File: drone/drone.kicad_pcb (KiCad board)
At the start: 2 copper layers, 50.8 x 50.8 mm, 28 parts, among them J1 Conn_01x03, J2 Conn_02x03_Top_Bottom, J3 Conn_01x02, J4 Conn_01x02, J5 Conn_01x02, J6 Conn_01x02, Q1 Si2319CDS, Q2 Si2319CDS, Q3 Si2319CDS, Q4 Si2319CDS, U1 ATmega328P-A, U2 MPU-6050, U3 DWM1000

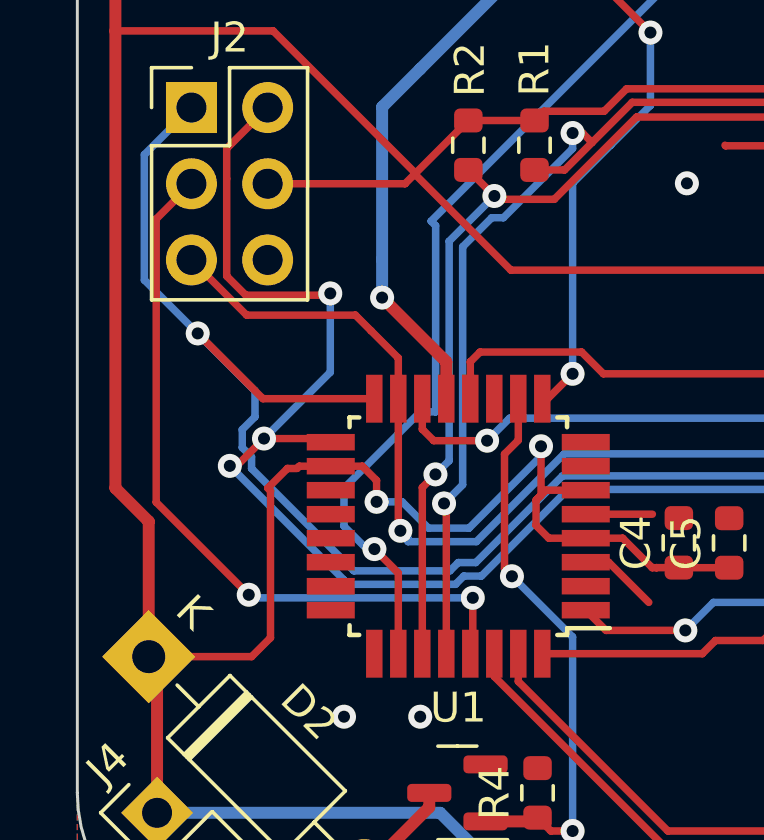
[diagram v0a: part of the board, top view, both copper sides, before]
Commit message: add reamde
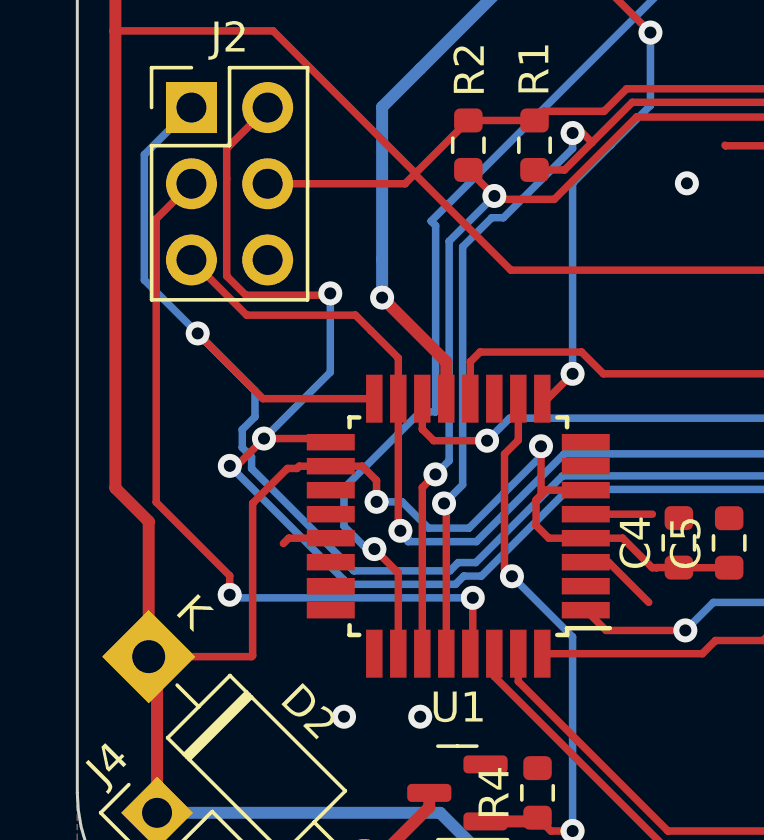
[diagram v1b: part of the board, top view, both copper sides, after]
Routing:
- net GND: track 14.3 -> 15.9 mm
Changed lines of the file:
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@@
   (segment (start 97.81 100.35) (end 97.79 100.33) (width 0.25) (layer "F.Cu") (net 36))
   (segment (start 93.15 112.63) (end 95.3702 112.63) (width 0.25) (layer "F.Cu") (net 36))
+  (segment (start 84.65 113.43) (end 83.246836 113.43) (width 0.25) (layer "F.Cu") (net 36))
   (segment (start 99.65 100.35) (end 97.81 100.35) (width 0.25) (layer "F.Cu") (net 36))
   (segment (start 100.825 105.41) (end 101.35 104.885) (width 0.25) (layer "F.Cu") (net 36))
   (segment (start 102.35 103.55) (end 102.35 104.040685) (width 0.25) (layer "F.Cu") (net 36))
+  (segment (start 83.246836 113.43) (end 83.068375 113.608461) (width 0.25) (layer "F.Cu") (net 36))
   (segment (start 103.15 106.4) (end 102.87 106.68) (width 0.25) (layer "F.Cu") (net 36))
   (segment (start 93.91 114.23) (end 95.25 115.57) (width 0.25) (layer "F.Cu") (net 36))
@@
   (segment (start 84.6328 107.8992) (end 82.423 110.109) (width 0.25) (layer "B.Cu") (net 38))
   (segment (start 89.3826 115.4176) (end 89.3826 117.1974) (width 0.25) (layer "F.Cu") (net 39))
-  (segment (start 78.83 102.79) (end 78.83 112.231) (width 0.25) (layer "F.Cu") (net 39))
-  (segment (start 78.83 112.231) (end 81.915 115.316) (width 0.25) (layer "F.Cu") (net 39))
   (segment (start 89.3826 117.1974) (end 89.3 117.28) (width 0.25) (layer "F.Cu") (net 39))
-  (segment (start 80.005 101.615) (end 78.83 102.79) (width 0.25) (layer "F.Cu") (net 39))
+  (segment (start 78.83 102.79) (end 80.005 101.615) (width 0.25) (layer "F.Cu") (net 39))
+  (segment (start 78.83 112.231) (end 78.83 102.79) (width 0.25) (layer "F.Cu") (net 39))
+  (segment (start 81.28 114.681) (end 78.83 112.231) (width 0.25) (layer "F.Cu") (net 39))
+  (segment (start 81.28 115.316) (end 81.28 114.681) (width 0.25) (layer "F.Cu") (net 39))
   (via (at 89.3826 115.4176) (size 0.8) (drill 0.4) (layers "F.Cu" "B.Cu") (net 39))
-  (via (at 81.915 115.316) (size 0.8) (drill 0.4) (layers "F.Cu" "B.Cu") (net 39))
-  (segment (start 82.0166 115.4176) (end 89.3826 115.4176) (width 0.25) (layer "B.Cu") (net 39))
-  (segment (start 81.915 115.316) (end 82.0166 115.4176) (width 0.25) (layer "B.Cu") (net 39))
+  (via (at 81.28 115.316) (size 0.8) (drill 0.4) (layers "F.Cu" "B.Cu") (net 39))
+  (segment (start 81.3816 115.4176) (end 89.3826 115.4176) (width 0.25) (layer "B.Cu") (net 39))
+  (segment (start 81.28 115.316) (end 81.3816 115.4176) (width 0.25) (layer "B.Cu") (net 39))
   (segment (start 117.390235 124.681275) (end 115.91896 123.21) (width 0.4) (layer "F.Cu") (net 40))
   (segment (start 103.55 102.85) (end 104.985 102.85) (width 0.25) (layer "F.Cu") (net 40))
@@
   (segment (start 90.6526 104.4956) (end 87.4739 101.3169) (width 0.25) (layer "F.Cu") (net 40))
   (segment (start 95.3638 114.4138) (end 94.38 113.43) (width 0.25) (layer "F.Cu") (net 40))
-  (segment (start 83.205 111.105) (end 82.55 111.76) (width 0.25) (layer "F.Cu") (net 40))
   (segment (start 91.656852 110.36615) (end 91.656852 112.000348) (width 0.25) (layer "F.Cu") (net 40))
+  (segment (start 82.044987 117.345013) (end 82.011634 117.378366) (width 0.25) (layer "F.Cu") (net 40))
   (segment (start 94.38 113.43) (end 93.15 113.43) (width 0.25) (layer "F.Cu") (net 40))
   (segment (start 117.057898 78.957898) (end 115.242492 77.142492) (width 0.4) (layer "F.Cu") (net 40))
   (segment (start 78.642492 80.760244) (end 78.837057 80.565679) (width 0.4) (layer "F.Cu") (net 40))
-  (segment (start 84.65 111.03) (end 83.6 111.03) (width 0.25) (layer "F.Cu") (net 40))
-  (segment (start 83.6 111.03) (end 83.525 111.105) (width 0.25) (layer "F.Cu") (net 40))
   (segment (start 91.8272 111.83) (end 91.4908 112.1664) (width 0.25) (layer "F.Cu") (net 40))
   (segment (start 106.167663 104.521) (end 105.8926 104.521) (width 0.25) (layer "F.Cu") (net 40))
@@
   (segment (start 119.6588 97.435) (end 119.6588 95.3) (width 0.25) (layer "F.Cu") (net 40))
   (segment (start 117.3557 79.2557) (end 117.057898 78.957898) (width 0.4) (layer "F.Cu") (net 40))
+  (segment (start 82.044987 112.265013) (end 82.044987 117.345013) (width 0.25) (layer "F.Cu") (net 40))
   (segment (start 78.580684 117.378366) (end 78.580684 112.870684) (width 0.4) (layer "F.Cu") (net 40))
   (segment (start 106.205996 97.975) (end 107.6706 99.439604) (width 0.25) (layer "F.Cu") (net 40))
+  (segment (start 83.205 111.105) (end 82.044987 112.265013) (width 0.25) (layer "F.Cu") (net 40))
   (segment (start 115.242492 77.142492) (end 80.337508 77.142492) (width 0.4) (layer "F.Cu") (net 40))
-  (segment (start 82.55 111.76) (end 82.64 111.85) (width 0.25) (layer "F.Cu") (net 40))
   (segment (start 77.47 96.52) (end 77.47 86.999189) (width 0.4) (layer "F.Cu") (net 40))
   (segment (start 100.85 104.3566) (end 100.711 104.4956) (width 0.25) (layer "F.Cu") (net 40))
-  (segment (start 82.64 111.85) (end 82.64 116.75) (width 0.25) (layer "F.Cu") (net 40))
-  (segment (start 82.011634 117.378366) (end 78.580684 117.378366) (width 0.25) (layer "F.Cu") (net 40))
   (segment (start 116.8588 95.3) (end 116.8588 97.6818) (width 0.25) (layer "F.Cu") (net 40))
   (segment (start 82.7278 96.52) (end 77.47 96.52) (width 0.25) (layer "F.Cu") (net 40))
   (segment (start 78.74 78.74) (end 78.837057 78.837057) (width 0.4) (layer "F.Cu") (net 40))
   (segment (start 122.644025 124.436286) (end 117.635224 124.436286) (width 0.4) (layer "F.Cu") (net 40))
-  (segment (start 83.525 111.105) (end 83.205 111.105) (width 0.25) (layer "F.Cu") (net 40))
   (segment (start 91.4908 113.0046) (end 91.9162 113.43) (width 0.25) (layer "F.Cu") (net 40))
+  (segment (start 83.6 111.03) (end 83.525 111.105) (width 0.25) (layer "F.Cu") (net 40))
   (segment (start 100.711 104.4956) (end 90.6526 104.4956) (width 0.25) (layer "F.Cu") (net 40))
   (segment (start 85.7 111.03) (end 86.1755 111.5055) (width 0.25) (layer "F.Cu") (net 40))
@@
   (segment (start 95.508205 114.409595) (end 95.504 114.4138) (width 0.25) (layer "F.Cu") (net 40))
   (segment (start 87.4739 101.3169) (end 87.4739 101.2661) (width 0.25) (layer "F.Cu") (net 40))
-  (segment (start 82.64 116.75) (end 82.011634 117.378366) (width 0.25) (layer "F.Cu") (net 40))
   (segment (start 91.656852 112.000348) (end 91.4908 112.1664) (width 0.25) (layer "F.Cu") (net 40))
   (segment (start 87.125 101.615) (end 87.4739 101.2661) (width 0.25) (layer "F.Cu") (net 40))
   (segment (start 78.580684 112.870684) (end 77.47 111.76) (width 0.4) (layer "F.Cu") (net 40))
+  (segment (start 82.011634 117.378366) (end 78.580684 117.378366) (width 0.25) (layer "F.Cu") (net 40))
   (segment (start 78.858992 117.656674) (end 78.580684 117.378366) (width 0.4) (layer "F.Cu") (net 40))
+  (segment (start 83.525 111.105) (end 83.205 111.105) (width 0.25) (layer "F.Cu") (net 40))
   (segment (start 116.6876 100.4062) (end 116.6876 100.457) (width 0.25) (layer "F.Cu") (net 40))
   (segment (start 101.522919 98.45) (end 101.997919 97.975) (width 0.25) (layer "F.Cu") (net 40))
@@
   (segment (start 100.85 103.55) (end 100.85 104.3566) (width 0.25) (layer "F.Cu") (net 40))
   (segment (start 106.68 125.73) (end 90.17 125.73) (width 0.4) (layer "F.Cu") (net 40))
+  (segment (start 84.65 111.03) (end 83.6 111.03) (width 0.25) (layer "F.Cu") (net 40))
   (segment (start 82.545 101.615) (end 87.125 101.615) (width 0.25) (layer "F.Cu") (net 40))
   (segment (start 101.997919 97.975) (end 106.205996 97.975) (width 0.25) (layer "F.Cu") (net 40))
